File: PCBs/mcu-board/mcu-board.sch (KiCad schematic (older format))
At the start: 7 parts, among them J1 ENCODER-PANEL-1, J2 ENCODER-PANEL-2, J3 5V, J4 3.3V, J5 MDAC-INPUT-SELECTOR, U1 m0-express

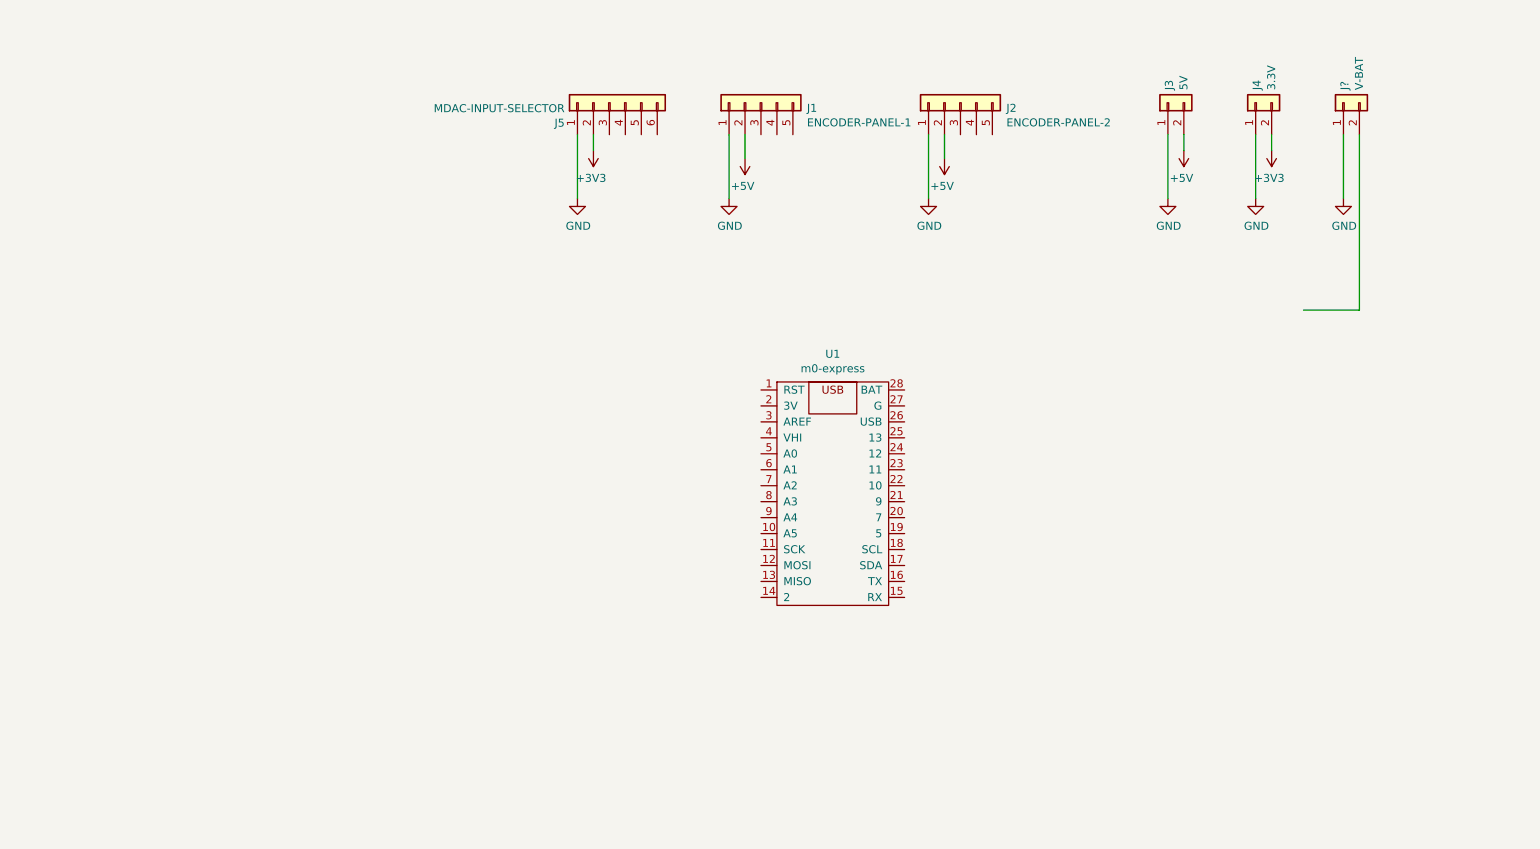
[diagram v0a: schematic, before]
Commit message: Updating mcu-board PCB
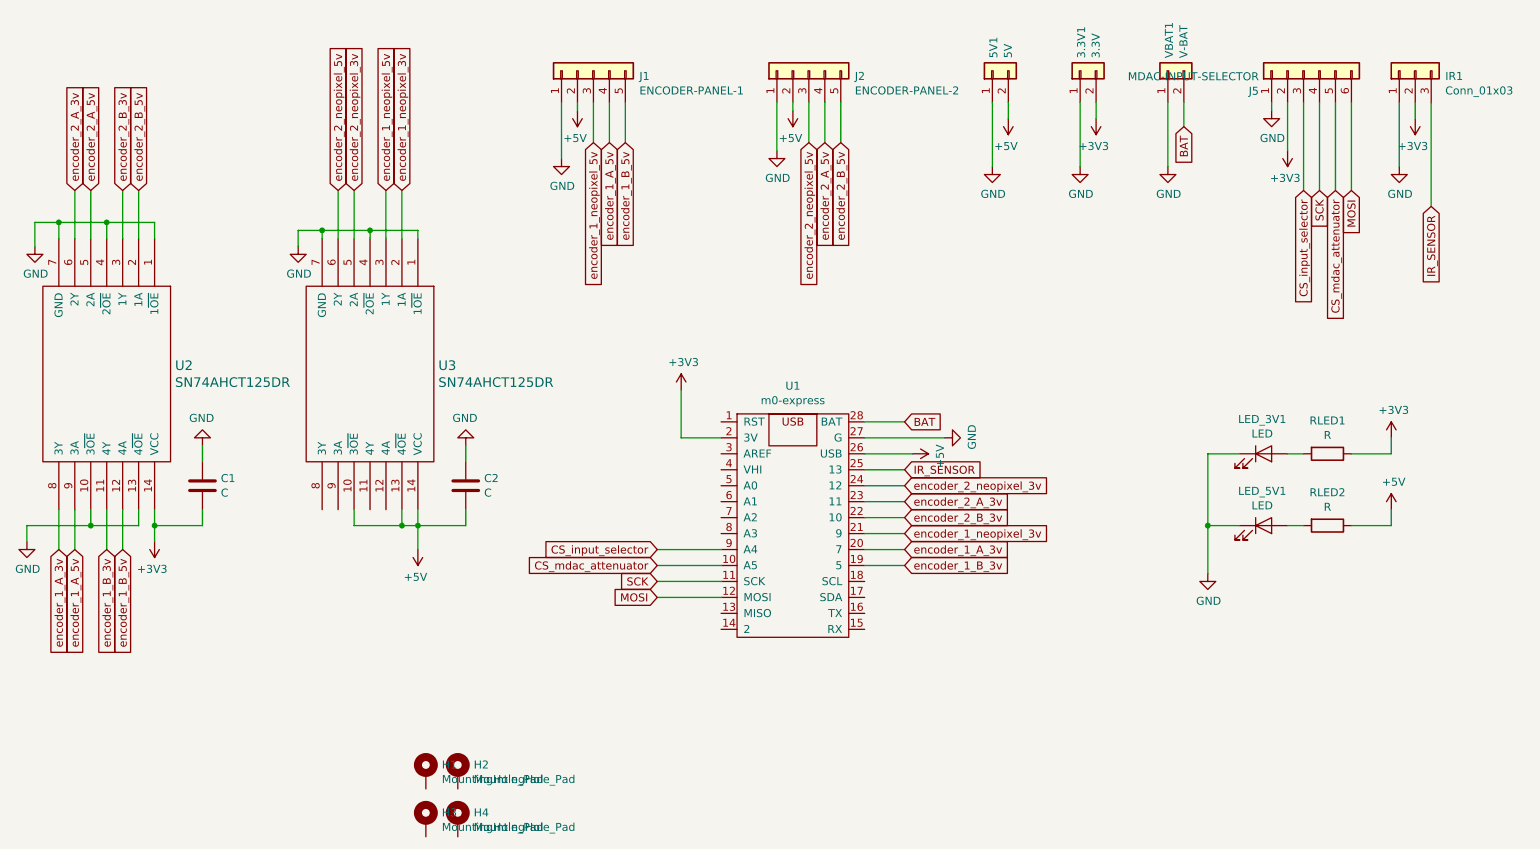
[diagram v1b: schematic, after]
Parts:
- added C1, C2: C, Capacitor_SMD:C_1206_3216Metric_Pad1.42x1.75mm_HandSolder, symbol Device:C
- added H1, H2, H3, H4: MountingHole_Pad, MountingHole:MountingHole_3.2mm_M3_Pad, symbol Mechanical:MountingHole_Pad
- added IR1: Conn_01x03, Connector_Molex:Molex_KK-254_AE-6410-03A_1x03_P2.54mm_Vertical, symbol Connector_Generic:Conn_01x03
- added LED_3V1, LED_5V1: LED, LED_SMD:LED_1206_3216Metric_Pad1.42x1.75mm_HandSolder, symbol Device:LED
- added RLED1, RLED2: R, Resistor_SMD:R_1206_3216Metric_Pad1.42x1.75mm_HandSolder, symbol Device:R
- added U2, U3: SN74AHCT125DR, Package_SO:SOIC-14_3.9x8.7mm_P1.27mm, symbol SN74AHCT125:SN74AHCT125
- gave numbers to parts that had none: 1
- renumbered J4 to 3.3V1, J3 to 5V1
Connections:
- net labels added: BAT, CS_input_selector, CS_mdac_attenuator, IR_SENSOR, MOSI, SCK, encoder_1_A_3v, encoder_1_A_5v, encoder_1_B_3v, encoder_1_B_5v, encoder_1_neopixel_3v, encoder_1_neopixel_5v, encoder_2_A_3v, encoder_2_A_5v, encoder_2_B_3v, encoder_2_B_5v, encoder_2_neopixel_3v, encoder_2_neopixel_5v
- wire segments 13 -> 96
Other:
- moved on the sheet: 3.3V1, 5V1, J1, J2, J5, U1, VBAT1
